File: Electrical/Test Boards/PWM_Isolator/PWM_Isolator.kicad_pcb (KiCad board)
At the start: 2 copper layers, 33.6 x 22 mm, 5 parts, among them P1 RC_HEADER, U1 SN74LVC1G34, U2 FOD817D3SD

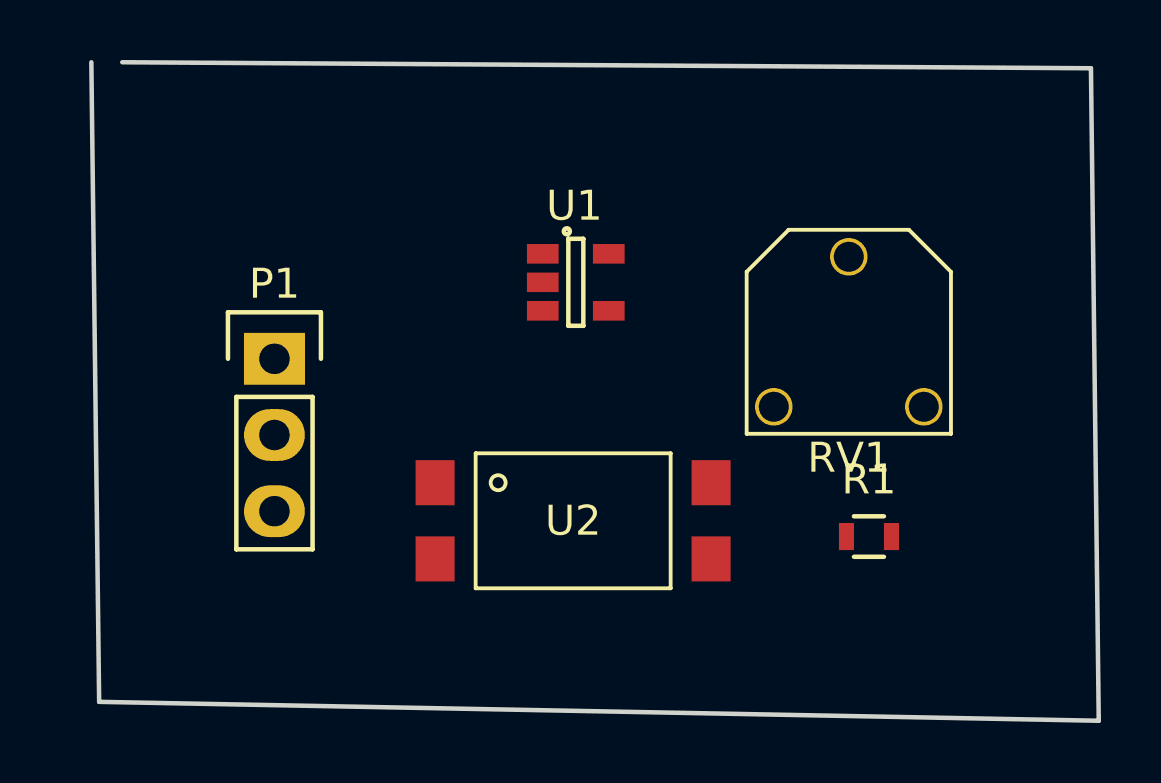
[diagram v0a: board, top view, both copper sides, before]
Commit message: PWM isolator updates
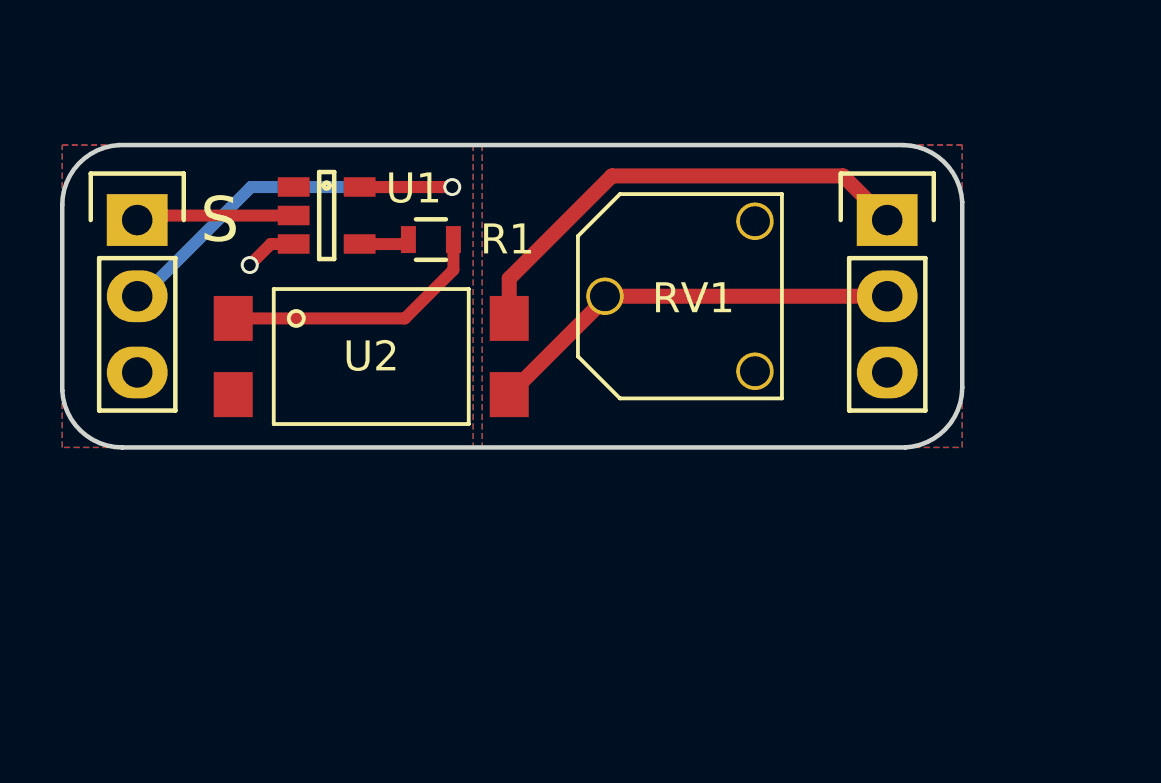
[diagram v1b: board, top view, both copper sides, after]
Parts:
- added P2: OUT_HEADER, Pin_Headers:Pin_Header_Straight_1x03, F.Cu at (165.0, 100.0)
- U1: footprint TO_SOT_Packages_SMD:SOT-23-5 -> pwm_isolator:SOT-23-5
- moved R1 17.6 mm to (149.8, 100.7), turned to 180 degrees
- moved U2 8.68 mm to (147.8, 104.5)
- moved U1 8.60 mm to (146.3, 99.8)
- moved P1 6.50 mm to (140.0, 100.0)
- moved RV1 4.83 mm to (160.6, 102.5), turned to 90 degrees
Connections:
- net /OUTPUT renamed Net-(P2-Pad2)
- P1 pad 3: GND -> GNDD
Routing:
- net +3V3: track 0.00 -> 16.0 mm
- net +5V: track 0.00 -> 15.1 mm, vias 0 -> 1
- net Net-(P2-Pad2): track 0.00 -> 14.0 mm
- net Net-(R1-Pad1): track 0.00 -> 9.02 mm
- net Net-(P1-Pad1): track 0.00 -> 5.28 mm
- net GNDD: track 0.00 -> 1.75 mm, vias 0 -> 1
- net Net-(R1-Pad2): track 0.00 -> 1.69 mm
- added copper zone on B.Cu, net GND
- added copper zone on F.Cu, net GND
- added copper zone on B.Cu, net GNDD
- added copper zone on F.Cu, net GNDD
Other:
- board size 33.6 x 22 mm -> 30 x 10.1 mm
- board text added: "3"
- board text added: "5"
- board text added: "Designed by Ops"
- board text added: "G"
- board text added: "NOCTIVORE"
- board text added: "S"
